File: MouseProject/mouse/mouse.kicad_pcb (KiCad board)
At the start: 2 copper layers, 60 x 102.5 mm, 66 parts, among them J1 B4B-PH-K-S_LF__SN_, J2 B02B-PASK-1, J3 B4B-PH-K-S_LF__SN_, J4 5051100492, J5 USB_B_Micro, J6 5051100492, Q7 MMBT3904-7-F, Q8 MMBT3904-7-F, Q9 MMBT3904-7-F, U1 AP2112K-3.3, U2 MIC5219-5.0YM5-TR, U3 TPS78319DDCT

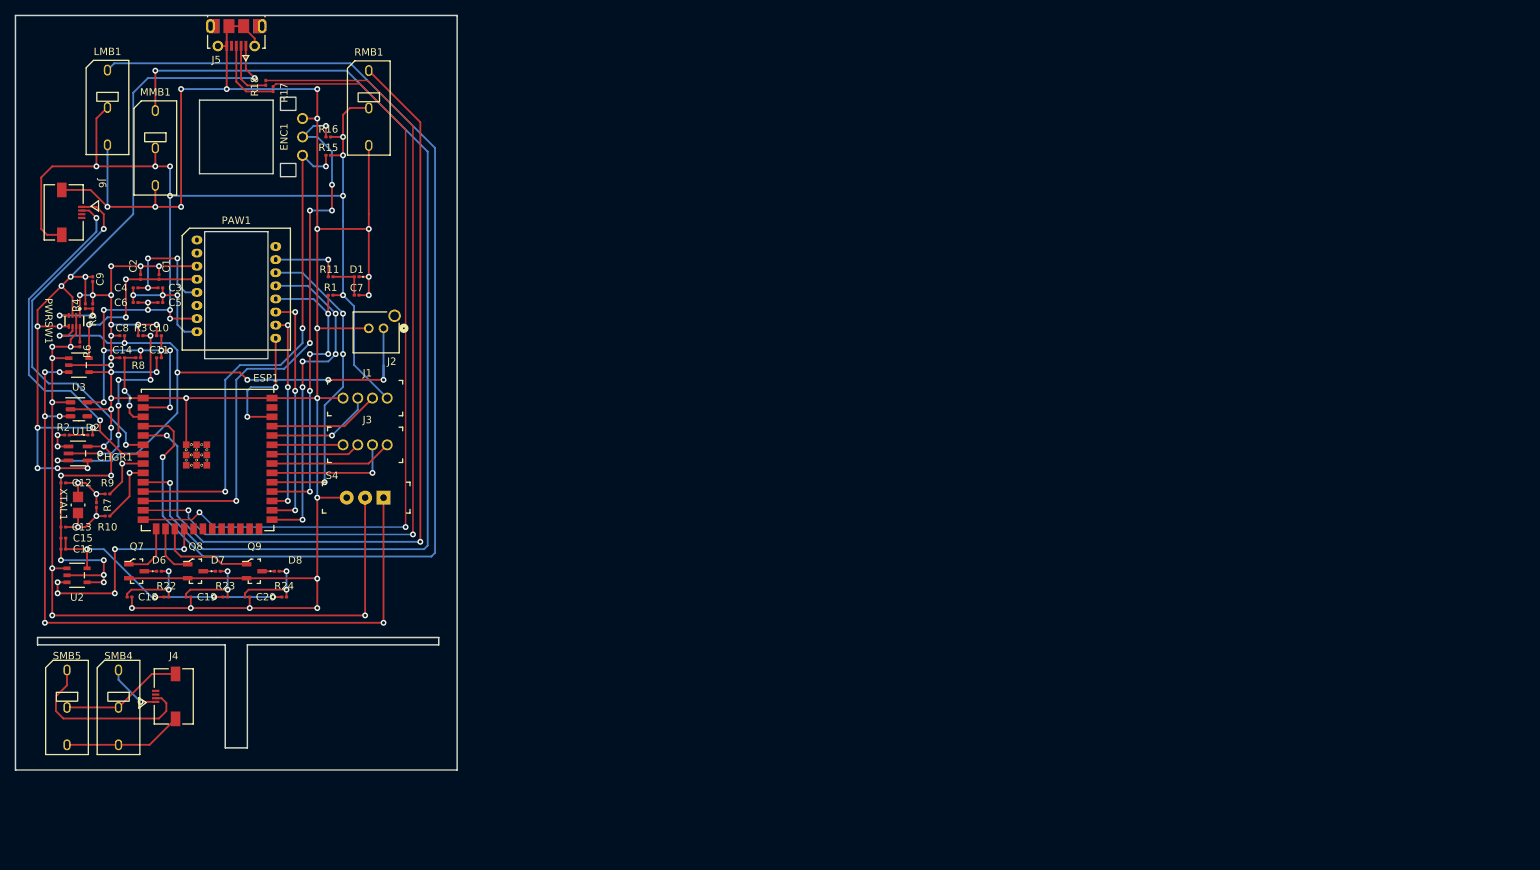
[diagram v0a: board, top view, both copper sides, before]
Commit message: Update for final board rev1
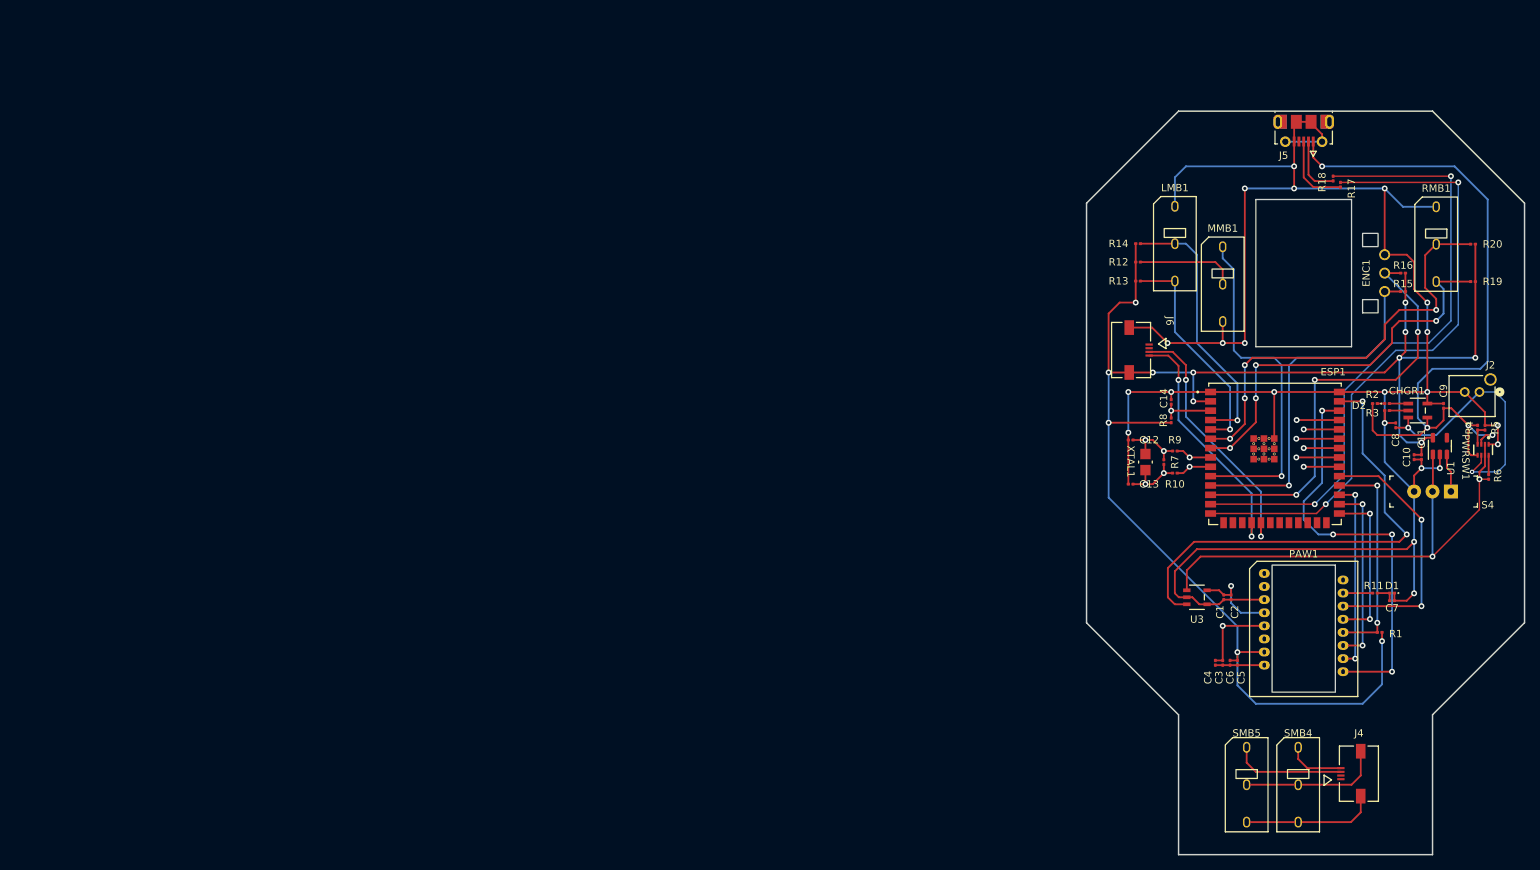
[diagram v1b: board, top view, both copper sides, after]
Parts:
- removed C15: 22uF, Capacitor_SMD:C_0201_0603Metric
- removed C16: 0.1uF, Capacitor_SMD:C_0201_0603Metric
- removed C18, C19, C20: 4.7uF, Capacitor_SMD:C_0201_0603Metric
- removed D6: LED_R, LED_SMD:LED_0201_0603Metric
- removed D7: LED_G, LED_SMD:LED_0201_0603Metric
- removed D8: LED_B, LED_SMD:LED_0201_0603Metric
- removed J1, J3: B4B-PH-K-S_LF__SN_, digikey-footprints:PinHeader_1x4_P2mm_Drill1mm
- removed Q7, Q8, Q9: MMBT3904-7-F, digikey-footprints:SOT-23-3
- removed R22, R23, R24: ??, Resistor_SMD:R_0201_0603Metric
- removed U2: MIC5219-5.0YM5-TR, MIC5219_5_0YM5_TR:SOT-23-5_M5_MCH
- added R12: 10k, Resistor_SMD:R_0201_0603Metric, F.Cu at (198.7, 54.0)
- added R13: 10k, Resistor_SMD:R_0201_0603Metric, F.Cu at (198.7, 56.5)
- added R14: 10k, Resistor_SMD:R_0201_0603Metric, F.Cu at (198.7, 51.5)
- added R19: 10k, Resistor_SMD:R_0201_0603Metric, F.Cu at (244.2, 56.6)
- added R20: 10k, Resistor_SMD:R_0201_0603Metric, F.Cu at (244.2, 51.5)
- moved R6 192.2 mm to (246.3, 83.1)
- moved PWRSW1 192.2 mm to (245.6, 79.5)
- moved R5 189.8 mm to (245.8, 76.5)
- moved R4 189.8 mm to (244.8, 76.5)
- moved U1 184.9 mm to (239.7, 79.0), turned to 90 degrees
- moved C9 184.3 mm to (240.2, 73.5), turned to -90 degrees
- moved CHGR1 182.1 mm to (236.7, 74.1)
- moved R2 179.4 mm to (232.5, 73.2), turned to 0 degrees
- moved D2 174.6 mm to (230.9, 73.2), turned to 180 degrees
- moved C8 173.4 mm to (233.7, 76.1), turned to -90 degrees
- moved C11 172.0 mm to (237.2, 80.5), turned to 90 degrees
- moved C10 171.3 mm to (236.2, 80.5), turned to 90 degrees
- moved R3 169.6 mm to (232.5, 74.1)
- moved J4 161.3 mm to (228.7, 123.5)
- moved SMB4 160.6 mm to (220.4, 119.9)
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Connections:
- ESP1 pad 18: PWR_5V_EN -> SW4_COM
- ESP1 pad 19: unconnected-(ESP1-IO11-Pad19) -> SW3_COM
- ESP1 pad 39: unconnected-(ESP1-IO1-Pad39) -> PWR_1.9V_EN
- ESP1 pad 4: SW1_COM -> SW1_NO
- ESP1 pad 5: SW2_COM -> SW1_NC
- ESP1 pad 6: SW3_COM -> SW2_NO
- ESP1 pad 7: SW4_COM -> SW2_NC
- J4 pad 1: SW3_COM_OFF -> unconnected-(J4-Pad1)
- J4 pad 2: SW4_COM_OFF -> unconnected-(J4-Pad2)
- J4 pad 3: unconnected-(J4-Pad3) -> SW4_COM_OFF
- J4 pad 4: unconnected-(J4-Pad4) -> SW3_COM_OFF
- J6 pad 1: SW3_COM -> unconnected-(J6-Pad1)
- J6 pad 2: SW4_COM -> unconnected-(J6-Pad2)
- J6 pad 3: unconnected-(J6-Pad3) -> SW3_COM
- J6 pad 4: unconnected-(J6-Pad4) -> SW4_COM
- LMB1 pad 1: SW1_COM -> GND
- LMB1 pad 2: PWR_3.3V -> SW1_NO
- LMB1 pad 3: GND -> SW1_NC
- MMB1 pad 2: PWR_3.3V -> SW5_NO
- RMB1 pad 1: SW2_COM -> GND
- RMB1 pad 2: PWR_3.3V -> SW2_NO
- RMB1 pad 3: GND -> SW2_NC
- U3 pad 3: PWR_EN -> PWR_1.9V_EN
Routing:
- net SW1_COM: track 160.7 -> 0.00 mm, vias 1 -> 0
- net SW2_COM: track 116.1 -> 0.00 mm, vias 2 -> 0
- net SCROLL_CLICK: track 145.7 -> 46.8 mm, vias 2 -> 1
- net PWR_EN: track 103.7 -> 5.26 mm, vias 6 -> 0
- net GND: track 408.8 -> 316.8 mm, vias 44 -> 22
- net PWR_1.9V_EN: track 0.00 -> 65.0 mm, vias 0 -> 2
- net SW2_NO: track 0.00 -> 58.7 mm, vias 0 -> 4
- net SW2_NC: track 0.00 -> 54.4 mm, vias 0 -> 4
- net +BATT: track 87.1 -> 35.8 mm, vias 7 -> 2
- net PWR_OUT: track 110.0 -> 70.1 mm, vias 7 -> 2
- net MOTION: track 17.6 -> 56.3 mm, vias 2 -> 4
- net PWR_5V: track 38.5 -> 0.00 mm, vias 4 -> 0
- net SW1_NO: track 0.00 -> 36.7 mm, vias 0 -> 1
- net USB_D-: track 116.7 -> 85.3 mm
- net SW1_NC: track 0.00 -> 30.6 mm, vias 0 -> 1
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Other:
- board size 60 x 102.5 mm -> 59.5 x 101 mm
